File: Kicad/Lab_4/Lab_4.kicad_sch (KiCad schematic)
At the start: 5 parts, among them SW1 SW_SPDT

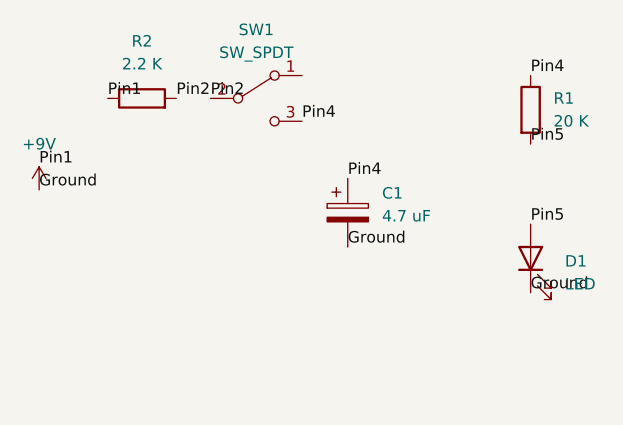
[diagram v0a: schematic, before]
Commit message: pcb design
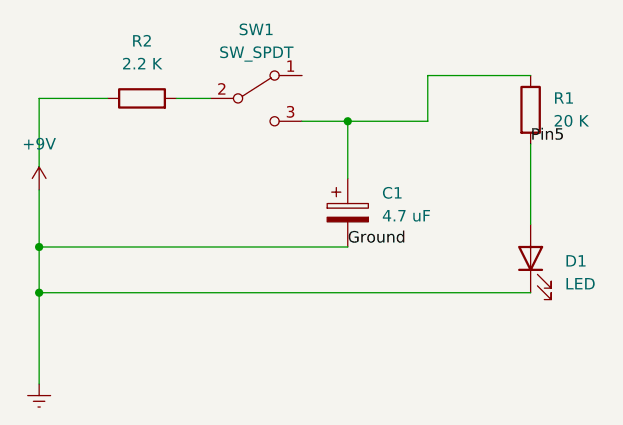
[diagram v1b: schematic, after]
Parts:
- C1: footprint (none) -> Capacitor_THT:C_Radial_D5.0mm_H5.0mm_P2.00mm
- D1: footprint (none) -> LED_THT:LED_D5.0mm
- R1, R2: footprint (none) -> Resistor_THT:R_Axial_DIN0516_L15.5mm_D5.0mm_P20.32mm_Horizontal
- SW1: footprint (none) -> Button_Switch_THT:SW_E-Switch_EG1224_SPDT_Angled
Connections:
- net Pin1: no longer names the net of R2.1
- net Pin2: no longer names the net of R2.2, SW1.2 (B)
- net Pin4: no longer names the net of C1.1, R1.1, SW1.3 (C)
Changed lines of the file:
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@@
 (kicad_sch (version 20211123) (generator eeschema)
   (paper "A4")
-  (label "Pin4" (at 95.25 92.71 0)
-    (effects (font (size 1.27 1.27)) (justify left bottom))
+  (junction (at 95.25 86.36) (diameter 0) (color 0 0 0 0)
   )
-  (label "Pin4" (at 115.57 81.28 0)
-    (effects (font (size 1.27 1.27)) (justify left bottom))
+  (junction (at 60.96 105.41) (diameter 0) (color 0 0 0 0)
+  )
+  (junction (at 60.96 100.33) (diameter 0) (color 0 0 0 0)
+  )
+  (wire (pts (xy 95.25 86.36) (xy 104.14 86.36))
+    (stroke (width 0) (type default) (color 0 0 0 0))
+  )
+  (wire (pts (xy 115.57 88.9) (xy 115.57 97.79))
+    (stroke (width 0) (type default) (color 0 0 0 0))
+  )
+  (wire (pts (xy 90.17 86.36) (xy 95.25 86.36))
+    (stroke (width 0) (type default) (color 0 0 0 0))
+  )
+  (wire (pts (xy 60.96 100.33) (xy 95.25 100.33))
+    (stroke (width 0) (type default) (color 0 0 0 0))
+  )
+  (wire (pts (xy 60.96 105.41) (xy 115.57 105.41))
+    (stroke (width 0) (type default) (color 0 0 0 0))
+  )
+  (wire (pts (xy 60.96 105.41) (xy 60.96 115.57))
+    (stroke (width 0) (type default) (color 0 0 0 0))
+  )
+  (wire (pts (xy 60.96 83.82) (xy 68.58 83.82))
+    (stroke (width 0) (type default) (color 0 0 0 0))
+  )
+  (wire (pts (xy 95.25 86.36) (xy 95.25 92.71))
+    (stroke (width 0) (type default) (color 0 0 0 0))
+  )
+  (wire (pts (xy 104.14 86.36) (xy 104.14 81.28))
+    (stroke (width 0) (type default) (color 0 0 0 0))
+  )
+  (wire (pts (xy 60.96 93.98) (xy 60.96 100.33))
+    (stroke (width 0) (type default) (color 0 0 0 0))
+  )
+  (wire (pts (xy 76.2 83.82) (xy 80.01 83.82))
+    (stroke (width 0) (type default) (color 0 0 0 0))
+  )
+  (wire (pts (xy 60.96 91.44) (xy 60.96 83.82))
+    (stroke (width 0) (type default) (color 0 0 0 0))
+  )
+  (wire (pts (xy 60.96 100.33) (xy 60.96 105.41))
+    (stroke (width 0) (type default) (color 0 0 0 0))
+  )
+  (wire (pts (xy 104.14 81.28) (xy 115.57 81.28))
+    (stroke (width 0) (type default) (color 0 0 0 0))
   )
   (label "Ground" (at 95.25 100.33 0)
     (effects (font (size 1.27 1.27)) (justify left bottom))
   )
-  (label "Pin5" (at 115.57 97.79 0)
-    (effects (font (size 1.27 1.27)) (justify left bottom))
-  )
-  (label "Ground" (at 60.96 93.98 0)
-    (effects (font (size 1.27 1.27)) (justify left bottom))
-  )
-  (label "Pin2" (at 80.01 83.82 0)
-    (effects (font (size 1.27 1.27)) (justify left bottom))
-  )
-  (label "Pin4" (at 90.17 86.36 0)
-    (effects (font (size 1.27 1.27)) (justify left bottom))
-  )
-  (label "Ground" (at 115.57 105.41 0)
-    (effects (font (size 1.27 1.27)) (justify left bottom))
-  )
   (label "Pin5" (at 115.57 88.9 0)
-    (effects (font (size 1.27 1.27)) (justify left bottom))
-  )
-  (label "Pin2" (at 76.2 83.82 0)
-    (effects (font (size 1.27 1.27)) (justify left bottom))
-  )
-  (label "Pin1" (at 60.96 91.44 0)
-    (effects (font (size 1.27 1.27)) (justify left bottom))
-  )
-  (label "Pin1" (at 68.58 83.82 0)
     (effects (font (size 1.27 1.27)) (justify left bottom))
   )
@@
     (property "Reference" "SW1" (id 0) (at 85.09 76.2 0))
     (property "Value" "SW_SPDT" (id 1) (at 85.09 78.74 0))
-    (property "Footprint" "" (id 2) (at 85.09 83.82 0)
+    (property "Footprint" "Button_Switch_THT:SW_E-Switch_EG1224_SPDT_Angled" (id 2) (at 85.09 83.82 0)
       (effects (font (size 1.27 1.27)) hide)
     )
@@
     (property "Reference" "R2" (id 0) (at 72.39 77.47 90))
     (property "Value" "2.2 K" (id 1) (at 72.39 80.01 90))
-    (property "Footprint" "" (id 2) (at 72.39 85.598 90)
+    (property "Footprint" "Resistor_THT:R_Axial_DIN0516_L15.5mm_D5.0mm_P20.32mm_Horizontal" (id 2) (at 72.39 85.598 90)
       (effects (font (size 1.27 1.27)) hide)
     )
@@
     )
     (property "Value" "+9V" (id 1) (at 60.96 88.9 0))
-    (property "Footprint" "" (id 2) (at 60.96 93.98 0)
+    (property "Footprint" "Connector_JST:JST_PH_B2B-PH-K_1x02_P2.00mm_Vertical" (id 2) (at 60.96 93.98 0)
       (effects (font (size 1.27 1.27)) hide)
     )
@@
       (effects (font (size 1.27 1.27)) (justify left))
     )
-    (property "Footprint" "" (id 2) (at 96.2152 100.33 0)
+    (property "Footprint" "Capacitor_THT:C_Radial_D5.0mm_H5.0mm_P2.00mm" (id 2) (at 96.2152 100.33 0)
       (effects (font (size 1.27 1.27)) hide)
     )
@@
       (effects (font (size 1.27 1.27)) (justify right))
     )
-    (property "Footprint" "" (id 2) (at 115.57 101.6 0)
+    (property "Footprint" "LED_THT:LED_D5.0mm" (id 2) (at 115.57 101.6 0)
       (effects (font (size 1.27 1.27)) hide)
     )
@@
       (effects (font (size 1.27 1.27)) (justify left))
     )
-    (property "Footprint" "" (id 2) (at 113.792 85.09 90)
+    (property "Footprint" "Resistor_THT:R_Axial_DIN0516_L15.5mm_D5.0mm_P20.32mm_Horizontal" (id 2) (at 113.792 85.09 90)
       (effects (font (size 1.27 1.27)) hide)
     )
@@
     (pin "2")
   )
+  (symbol (lib_id "power:Earth") (at 60.96 115.57 0) (unit 1)
+    (in_bom yes) (on_board yes) (fields_autoplaced)
+    (property "Reference" "#PWR0101" (id 0) (at 60.96 121.92 0)
+      (effects (font (size 1.27 1.27)) hide)
+    )
+    (property "Value" "Earth" (id 1) (at 60.96 119.38 0)
+      (effects (font (size 1.27 1.27)) hide)
+    )
+    (property "Footprint" "" (id 2) (at 60.96 115.57 0)
+      (effects (font (size 1.27 1.27)) hide)
+    )
+    (property "Datasheet" "~" (id 3) (at 60.96 115.57 0)
+      (effects (font (size 1.27 1.27)) hide)
+    )
+    (pin "1")
+  )
   (sheet_instances
     (path "/" (page "1"))
@@
   (symbol_instances
     (path "/2d110ae4-e4fc-48ee-a5f2-dab5634b50d1"
-      (reference "#PWR01") (unit 1) (value "+9V") (footprint "")
+      (reference "#PWR01") (unit 1) (value "+9V") (footprint "Connector_JST:JST_PH_B2B-PH-K_1x02_P2.00mm_Vertical")
+    )
+    (path "/e552c34d-4b7d-45a2-9e9a-60cb47d5f1e3"
+      (reference "#PWR0101") (unit 1) (value "Earth") (footprint "")
     )
     (path "/48d5f641-1232-4ccf-baa8-19a3a249d553"
-      (reference "C1") (unit 1) (value "4.7 uF") (footprint "")
+      (reference "C1") (unit 1) (value "4.7 uF") (footprint "Capacitor_THT:C_Radial_D5.0mm_H5.0mm_P2.00mm")
     )
     (path "/5994e999-6f61-4b13-a2ae-b2b151ba44ac"
-      (reference "D1") (unit 1) (value "LED") (footprint "")
+      (reference "D1") (unit 1) (value "LED") (footprint "LED_THT:LED_D5.0mm")
     )
     (path "/d5474086-ea55-48ec-8447-baa91e59b827"
-      (reference "R1") (unit 1) (value "20 K") (footprint "")
+      (reference "R1") (unit 1) (value "20 K") (footprint "Resistor_THT:R_Axial_DIN0516_L15.5mm_D5.0mm_P20.32mm_Horizontal")
     )
     (path "/19c3e5cb-fc1a-4cfd-89fe-ea154dcc5741"
-      (reference "R2") (unit 1) (value "2.2 K") (footprint "")
+      (reference "R2") (unit 1) (value "2.2 K") (footprint "Resistor_THT:R_Axial_DIN0516_L15.5mm_D5.0mm_P20.32mm_Horizontal")
     )
     (path "/14e300eb-e30d-4e67-bace-ae7d4adbb157"
-      (reference "SW1") (unit 1) (value "SW_SPDT") (footprint "")
+      (reference "SW1") (unit 1) (value "SW_SPDT") (footprint "Button_Switch_THT:SW_E-Switch_EG1224_SPDT_Angled")
     )
   )
